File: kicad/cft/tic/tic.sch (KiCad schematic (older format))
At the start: 14 parts, among them U24 AMS1117-3.3, U40 8254

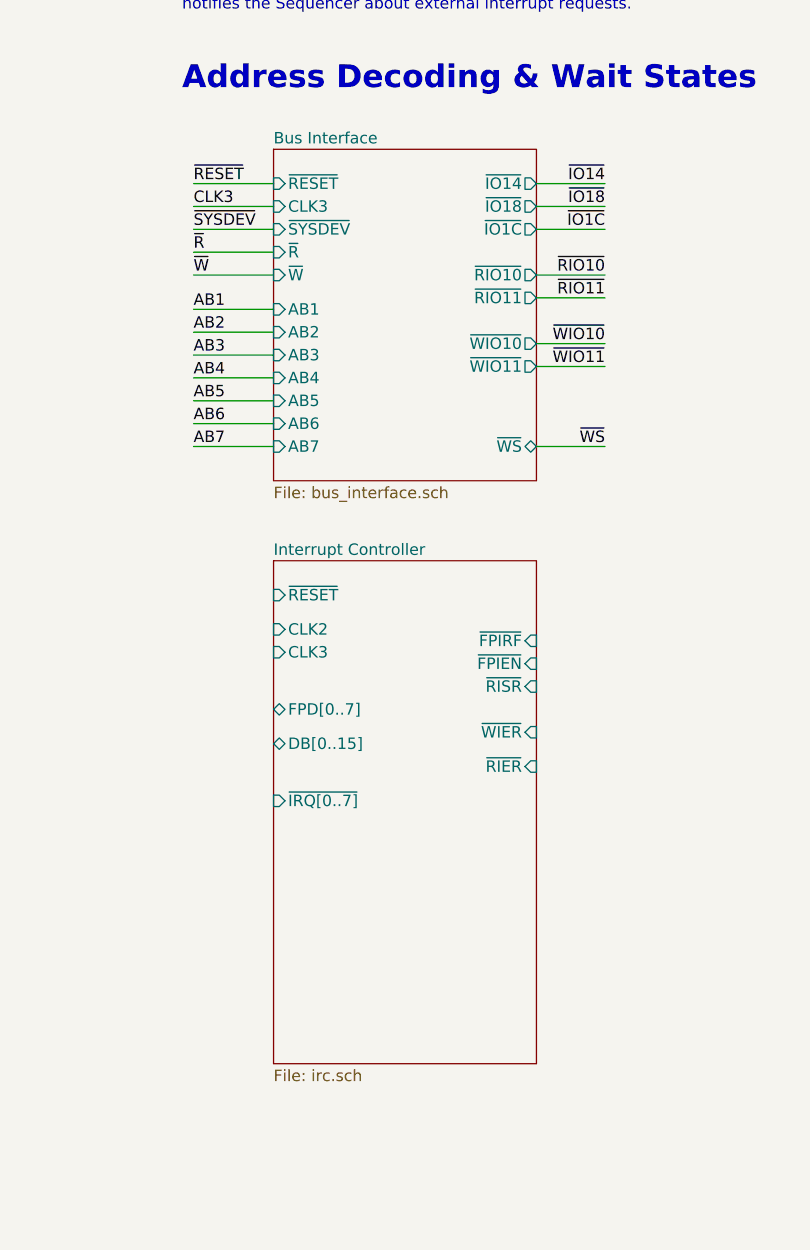
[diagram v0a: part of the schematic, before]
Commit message: Minor changes.
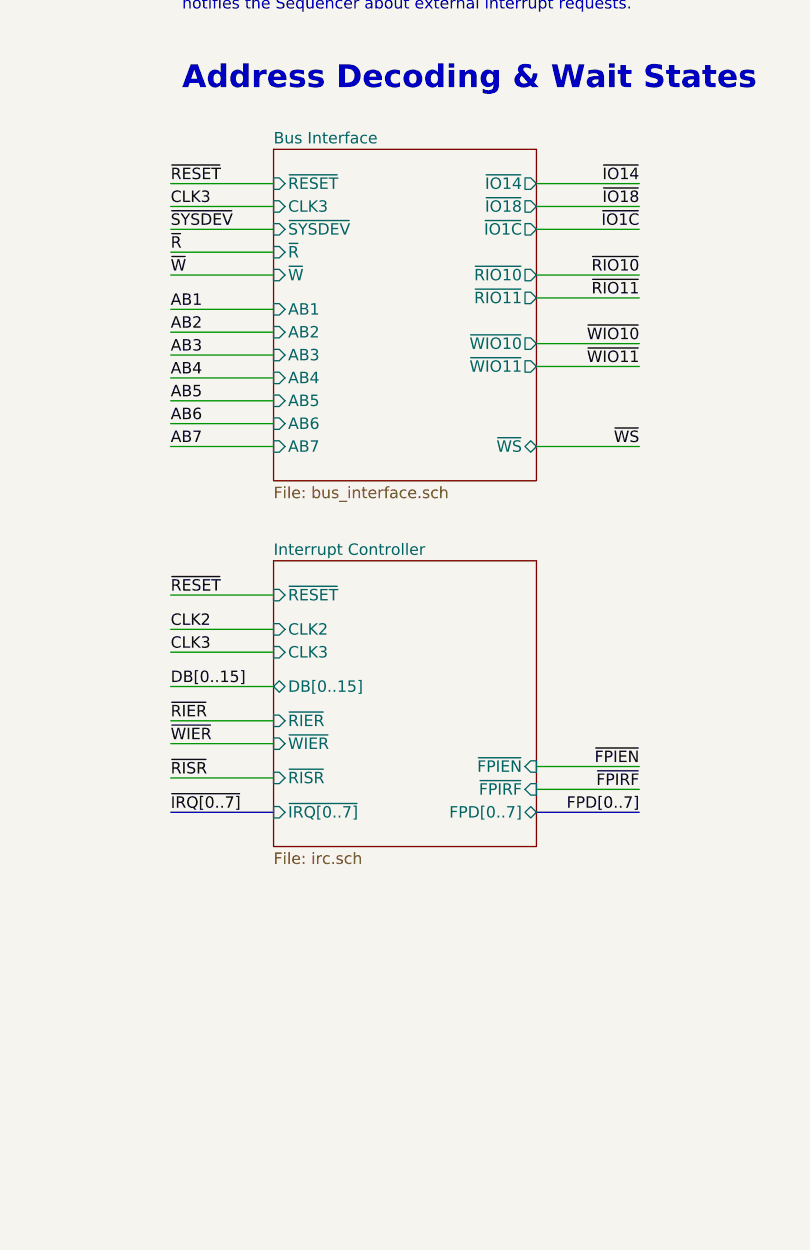
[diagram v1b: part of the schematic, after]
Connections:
- net labels added: ~FPIEN, ~FPIRF, ~RIER, ~RISR, ~WIER
- wire segments 132 -> 141
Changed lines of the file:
@@
 $EndSheet
 Wire Wire Line
-	1100 2400 750  2400
+	1100 2400 650  2400
 Wire Wire Line
-	1100 2500 750  2500
+	1100 2500 650  2500
 Wire Wire Line
-	1100 2600 750  2600
+	1100 2600 650  2600
 Wire Wire Line
-	1100 2700 750  2700
+	1100 2700 650  2700
 Wire Wire Line
-	1100 2800 750  2800
+	1100 2800 650  2800
 Wire Wire Line
-	750  2950 1100 2950
+	650  2950 1100 2950
 Wire Wire Line
-	750  3050 1100 3050
+	650  3050 1100 3050
 Wire Wire Line
-	750  3150 1100 3150
+	650  3150 1100 3150
 Wire Wire Line
-	750  3250 1100 3250
+	650  3250 1100 3250
 Wire Wire Line
-	750  3350 1100 3350
+	650  3350 1100 3350
 Wire Wire Line
-	750  3450 1100 3450
+	650  3450 1100 3450
 Wire Wire Line
-	750  3550 1100 3550
+	650  3550 1100 3550
 Wire Wire Line
-	2550 2400 2250 2400
+	2700 2400 2250 2400
 Wire Wire Line
-	2550 2500 2250 2500
+	2700 2500 2250 2500
 Wire Wire Line
-	2550 2600 2250 2600
+	2700 2600 2250 2600
 Wire Wire Line
-	2550 2800 2250 2800
+	2700 2800 2250 2800
 Wire Wire Line
-	2250 2900 2550 2900
+	2250 2900 2700 2900
 Wire Wire Line
-	2250 3100 2550 3100
+	2250 3100 2700 3100
 Wire Wire Line
-	2250 3200 2550 3200
+	2250 3200 2700 3200
 Wire Wire Line
-	2250 3550 2550 3550
+	2250 3550 2700 3550
 Text Notes 700  2000 0    100  ~ 20
 Address Decoding & Wait States
-Text Label 750  2400 0    50   ~ 0
+Text Label 650  2400 0    50   ~ 0
 ~RESET
-Text Label 750  2500 0    50   ~ 0
+Text Label 650  2500 0    50   ~ 0
 CLK3
-Text Label 750  2600 0    50   ~ 0
+Text Label 650  2600 0    50   ~ 0
 ~SYSDEV
-Text Label 750  2700 0    50   ~ 0
+Text Label 650  2700 0    50   ~ 0
 ~R
-Text Label 750  2800 0    50   ~ 0
+Text Label 650  2800 0    50   ~ 0
 ~W
-Text Label 750  2950 0    50   ~ 0
+Text Label 650  2950 0    50   ~ 0
 AB1
-Text Label 750  3050 0    50   ~ 0
+Text Label 650  3050 0    50   ~ 0
 AB2
-Text Label 750  3150 0    50   ~ 0
+Text Label 650  3150 0    50   ~ 0
 AB3
-Text Label 750  3250 0    50   ~ 0
+Text Label 650  3250 0    50   ~ 0
 AB4
-Text Label 750  3350 0    50   ~ 0
+Text Label 650  3350 0    50   ~ 0
 AB5
-Text Label 750  3450 0    50   ~ 0
+Text Label 650  3450 0    50   ~ 0
 AB6
-Text Label 750  3550 0    50   ~ 0
+Text Label 650  3550 0    50   ~ 0
 AB7
-Text Label 2550 2400 2    50   ~ 0
+Text Label 2700 2400 2    50   ~ 0
 ~IO14
-Text Label 2550 2500 2    50   ~ 0
+Text Label 2700 2500 2    50   ~ 0
 ~IO18
-Text Label 2550 2600 2    50   ~ 0
+Text Label 2700 2600 2    50   ~ 0
 ~IO1C
-Text Label 2550 2800 2    50   ~ 0
+Text Label 2700 2800 2    50   ~ 0
 ~RIO10
-Text Label 2550 2900 2    50   ~ 0
+Text Label 2700 2900 2    50   ~ 0
 ~RIO11
-Text Label 2550 3100 2    50   ~ 0
+Text Label 2700 3100 2    50   ~ 0
 ~WIO10
-Text Label 2550 3200 2    50   ~ 0
+Text Label 2700 3200 2    50   ~ 0
 ~WIO11
-Text Label 2550 3550 2    50   ~ 0
+Text Label 2700 3550 2    50   ~ 0
 ~WS
 $Sheet
-S 1100 4050 1150 2200
+S 1100 4050 1150 1250
 U 5F160E7C
 F0 "Interrupt Controller" 50
 F1 "irc.sch" 50
-F2 "DB[0..15]" T L 1100 4850 50
-F3 "~RIER" I R 2250 4950 50
-F4 "FPD[0..7]" T L 1100 4700 50
+F2 "DB[0..15]" T L 1100 4600 50
+F3 "~RIER" I L 1100 4750 50
+F4 "FPD[0..7]" T R 2250 5150 50
 F5 "CLK3" I L 1100 4450 50
 F6 "CLK2" I L 1100 4350 50
 F7 "~RESET" I L 1100 4200 50
-F8 "~WIER" I R 2250 4800 50
-F9 "~IRQ[0..7]" I L 1100 5100 50
-F10 "~RISR" I R 2250 4600 50
-F11 "~FPIEN" I R 2250 4500 50
-F12 "~FPIRF" I R 2250 4400 50
+F8 "~WIER" I L 1100 4850 50
+F9 "~IRQ[0..7]" I L 1100 5150 50
+F10 "~RISR" I L 1100 5000 50
+F11 "~FPIEN" I R 2250 4950 50
+F12 "~FPIRF" I R 2250 5050 50
 $EndSheet
+Wire Bus Line
+	1100 5150 650  5150
+Wire Wire Line
+	1100 4200 650  4200
+Wire Wire Line
+	1100 4350 650  4350
+Wire Wire Line
+	1100 4450 650  4450
+Wire Wire Line
+	1100 4600 650  4600
+Wire Wire Line
+	1100 4750 650  4750
+Wire Wire Line
+	1100 4850 650  4850
+Wire Wire Line
+	1100 5000 650  5000
+Wire Wire Line
+	2250 4950 2700 4950
+Wire Wire Line
+	2250 5050 2700 5050
+Wire Bus Line
+	2700 5150 2250 5150
+Text Label 2700 4950 2    50   ~ 0
+~FPIEN
+Text Label 2700 5050 2    50   ~ 0
+~FPIRF
+Text Label 650  5150 0    50   ~ 0
+~IRQ[0..7]
+Text Label 650  4200 0    50   ~ 0
+~RESET
+Text Label 650  4350 0    50   ~ 0
+CLK2
+Text Label 650  4450 0    50   ~ 0
+CLK3
+Text Label 650  4600 0    50   ~ 0
+DB[0..15]
+Text Label 650  4750 0    50   ~ 0
+~RIER
+Text Label 650  4850 0    50   ~ 0
+~WIER
+Text Label 650  5000 0    50   ~ 0
+~RISR
+Text Label 2700 5150 2    50   ~ 0
+FPD[0..7]
 $EndSCHEMATC
